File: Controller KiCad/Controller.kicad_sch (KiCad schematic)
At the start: 11 parts, among them J1 ESP32 L-Header, J2 ESP32 R-Header, J3 Conn_01x05, SW1 SW_Push, SW2 SW_Push, SW3 SW_Push, SW4 SW_Push

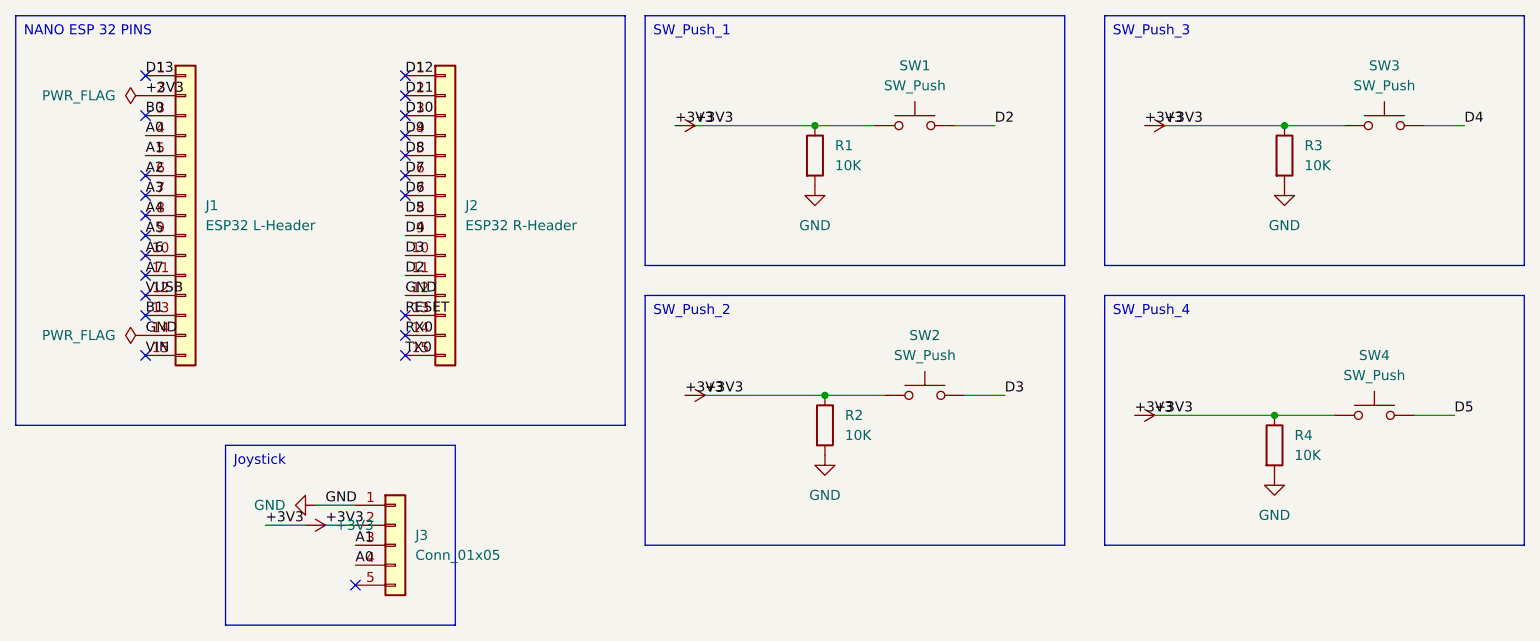
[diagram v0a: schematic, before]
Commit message: Almost complete PCB
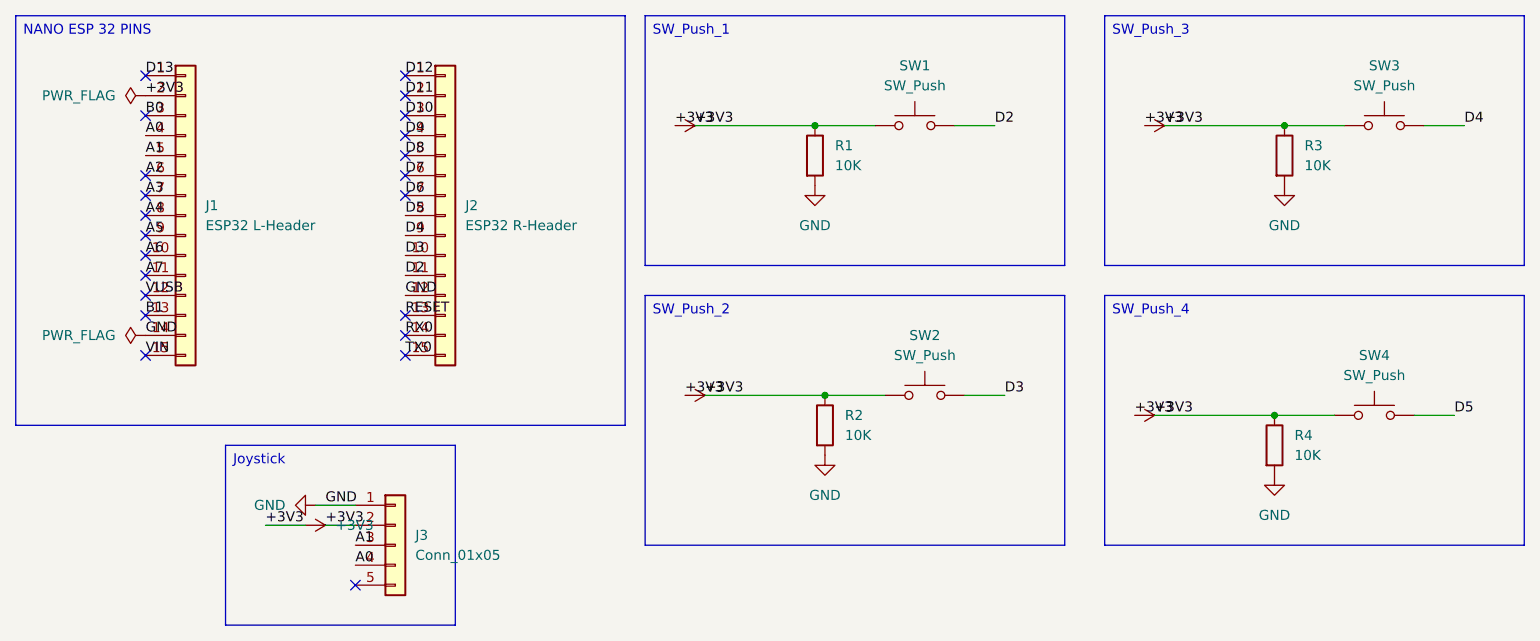
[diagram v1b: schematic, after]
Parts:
- J1, J2: footprint (none) -> Connector_PinHeader_2.54mm:PinHeader_1x15_P2.54mm_Vertical
- J3: footprint (none) -> Connector_PinHeader_2.54mm:PinHeader_1x05_P2.54mm_Vertical
- R1, R2, R3, R4: footprint (none) -> Resistor_THT:R_Axial_DIN0207_L6.3mm_D2.5mm_P7.62mm_Horizontal
- SW1, SW2, SW3, SW4: footprint (none) -> Button_Switch_THT:SW_PUSH_6mm
